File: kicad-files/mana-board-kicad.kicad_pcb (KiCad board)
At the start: 2 copper layers, 155.5 x 110 mm, 44 parts, among them U1 Pico

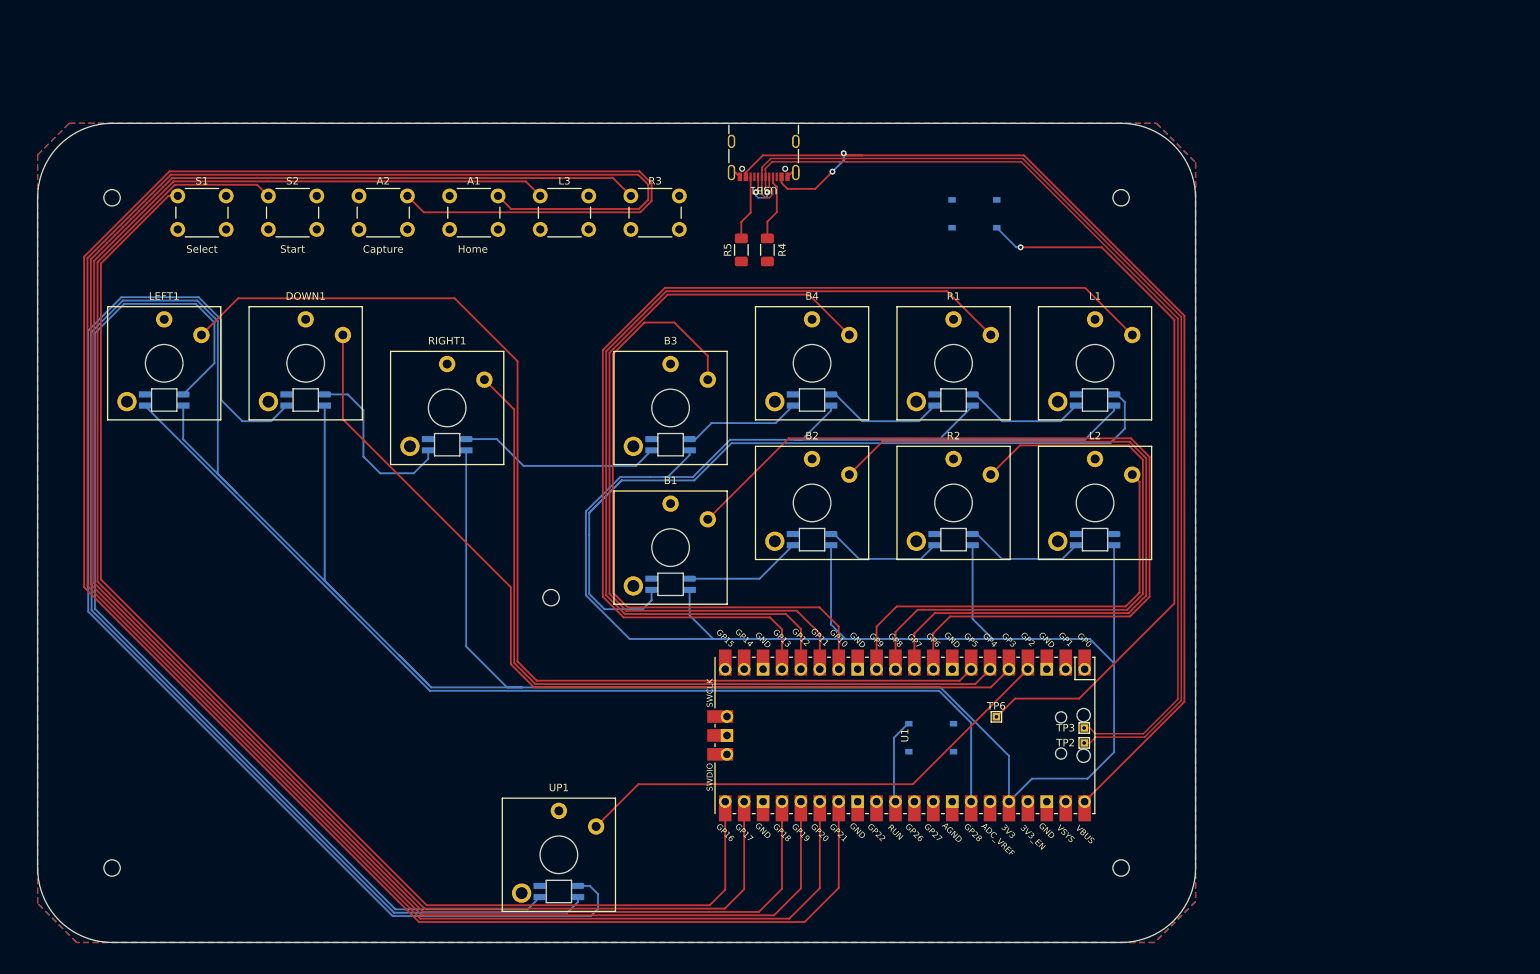
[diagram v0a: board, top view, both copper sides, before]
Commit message: Organize libraries, start rev1
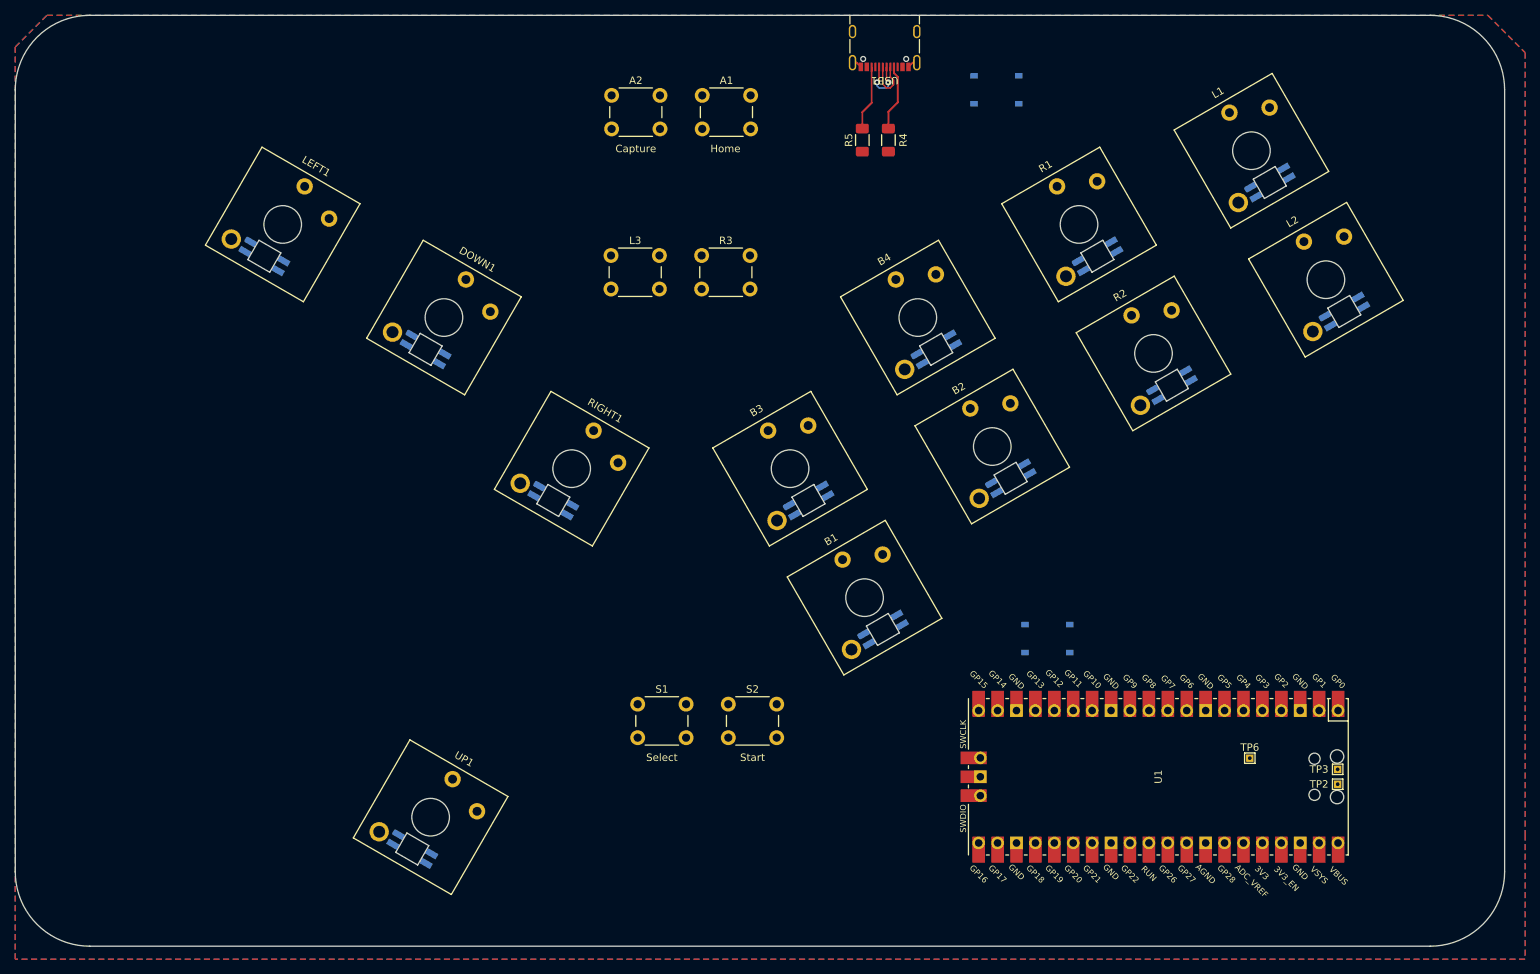
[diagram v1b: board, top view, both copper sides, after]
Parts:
- removed REF** (x5): MountingHole_2.2mm_M2, MountingHole:MountingHole_2.2mm_M2
- B1, B2, B3, B4, DOWN1, L1, L2, LEFT1, R1, R2, RIGHT1, UP1: footprint Switch_Keyboard_Kailh:SW_Kailh_Choc_V2_1.00u -> ManaBoard:SW_Kailh_Choc_V2
- D1: value SK6812MINI -> SK6812MINI-E; footprint Footprints:SK6812-MINI-E-reversed -> ManaBoard:SK6812-MINI-E
- D10, D11, D12, D2, D3, D4, D5, D6, D7, D8, D9: footprint Footprints:SK6812-MINI-E-reversed -> ManaBoard:SK6812-MINI-E
- R4, R5: value R_Small -> 5.1k
- TP2: value TestPoint -> PI DM
- TP3: value TestPoint -> PI DP
- moved S1 92.0 mm to (139.3, 125.5)
- moved S2 92.0 mm to (151.5, 125.5)
- moved D12 45.4 mm to (234.2, 72.8), turned to -150 degrees
- moved L2 43.1 mm to (231.8, 68.5), turned to 30 degrees
- moved D8 37.5 mm to (224.2, 55.4), turned to -150 degrees
- moved A2 36.5 mm to (135.8, 43.8)
- moved A1 36.5 mm to (148.0, 43.8)
- moved D11 35.9 mm to (211.1, 82.7), turned to -150 degrees
- moved L1 35.4 mm to (221.8, 51.2), turned to 30 degrees
- moved TP2 34.5 mm to (233.3, 136.2)
- moved TP3 34.5 mm to (233.3, 134.2)
- moved TP6 34.5 mm to (221.5, 132.8)
- moved U1 34.5 mm to (209.2, 135.2)
- moved R2 33.5 mm to (208.6, 78.4), turned to 30 degrees
- moved D9 29.2 mm to (172.3, 115.5), turned to -150 degrees
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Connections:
- D1 pad 1: Net-(D1-DOUT) -> 5V
- D1 pad 2: GND -> Net-(D1-DOUT)
- D1 pad 3: Net-(D1-DIN) -> GND
- D1 pad 4: Net-(D1-VDD) -> RGBDATA
- D10 pad 1: Net-(D10-DOUT) -> 5V
- D10 pad 2: GND -> Net-(D10-DOUT)
- D10 pad 3: Net-(D10-DIN) -> GND
- D10 pad 4: Net-(D1-VDD) -> Net-(D10-DIN)
- D11 pad 1: Net-(D11-DOUT) -> 5V
- D11 pad 2: GND -> Net-(D11-DOUT)
- D11 pad 3: Net-(D10-DOUT) -> GND
- D11 pad 4: Net-(D1-VDD) -> Net-(D10-DOUT)
- D12 pad 1: unconnected-(D12-DOUT-Pad1) -> 5V
- D12 pad 2: GND -> unconnected-(D12-DOUT-Pad2)
- D12 pad 3: Net-(D11-DOUT) -> GND
- D12 pad 4: Net-(D1-VDD) -> Net-(D11-DOUT)
- D2 pad 1: Net-(D2-DOUT) -> 5V
- D2 pad 2: GND -> Net-(D2-DOUT)
- D2 pad 3: Net-(D1-DOUT) -> GND
- D2 pad 4: Net-(D1-VDD) -> Net-(D1-DOUT)
- D3 pad 1: Net-(D3-DOUT) -> 5V
- D3 pad 2: GND -> Net-(D3-DOUT)
- D3 pad 3: Net-(D2-DOUT) -> GND
- D3 pad 4: Net-(D1-VDD) -> Net-(D2-DOUT)
- D4 pad 1: Net-(D4-DOUT) -> 5V
- D4 pad 2: GND -> Net-(D4-DOUT)
- D4 pad 3: Net-(D3-DOUT) -> GND
- D4 pad 4: Net-(D1-VDD) -> Net-(D3-DOUT)
- D5 pad 1: Net-(D5-DOUT) -> 5V
- D5 pad 2: GND -> Net-(D5-DOUT)
- D5 pad 3: Net-(D4-DOUT) -> GND
- D5 pad 4: Net-(D1-VDD) -> Net-(D4-DOUT)
- D6 pad 1: Net-(D6-DOUT) -> 5V
- D6 pad 2: GND -> Net-(D6-DOUT)
- D6 pad 3: Net-(D5-DOUT) -> GND
- D6 pad 4: Net-(D1-VDD) -> Net-(D5-DOUT)
- D7 pad 1: Net-(D7-DOUT) -> 5V
- D7 pad 2: GND -> Net-(D7-DOUT)
- D7 pad 3: Net-(D6-DOUT) -> GND
- D7 pad 4: Net-(D1-VDD) -> Net-(D6-DOUT)
- D8 pad 1: Net-(D8-DOUT) -> 5V
- D8 pad 2: GND -> Net-(D8-DOUT)
- D8 pad 3: Net-(D7-DOUT) -> GND
- D8 pad 4: Net-(D1-VDD) -> Net-(D7-DOUT)
- D9 pad 1: Net-(D10-DIN) -> 5V
- D9 pad 2: GND -> Net-(D10-DIN)
- D9 pad 3: Net-(D8-DOUT) -> GND
- D9 pad 4: Net-(D1-VDD) -> Net-(D8-DOUT)
- U1 pad 28: GND -> unconnected-(U1-GND-Pad28)
- U1 pad 34: Net-(D1-DIN) -> RGBDATA
- U1 pad 36: Net-(D1-VDD) -> 3.3V
- U1 pad 40: Net-(U1-VBUS) -> 5V
- USB1 pad A4: Net-(U1-VBUS) -> 5V
- USB1 pad A9: Net-(U1-VBUS) -> 5V
- USB1 pad B4: Net-(U1-VBUS) -> 5V
- USB1 pad B9: Net-(U1-VBUS) -> 5V
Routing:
- net Net-(D1-VDD): track 639.6 -> 0.00 mm
- net Net-(U1-GPIO21): track 296.1 -> 0.00 mm
- net Net-(U1-GPIO20): track 278.1 -> 0.00 mm
- net Net-(U1-GPIO19): track 248.6 -> 0.00 mm
- net Net-(U1-GPIO18): track 232.0 -> 0.00 mm
- net Net-(U1-GPIO17): track 188.6 -> 0.00 mm
- net Net-(D2-DOUT): track 171.3 -> 0.00 mm
- net Net-(U1-GPIO16): track 171.1 -> 0.00 mm
- net Net-(U1-VBUS): track 154.8 -> 0.00 mm, vias 2 -> 0
- net Net-(U1-GPIO5): track 150.9 -> 0.00 mm
- net Net-(D1-DOUT): track 144.3 -> 0.00 mm
- net Net-(U1-GPIO13): track 141.5 -> 0.00 mm
- net Net-(D1-DIN): track 139.2 -> 0.00 mm
- net /Pi D-: track 141.0 -> 7.18 mm
- net /Pi D+: track 139.1 -> 7.54 mm
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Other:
- board size 155.5 x 110 mm -> 200 x 125 mm
